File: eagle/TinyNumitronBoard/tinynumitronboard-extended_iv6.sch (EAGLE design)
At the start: 50 parts, among them IC1 74LS595D

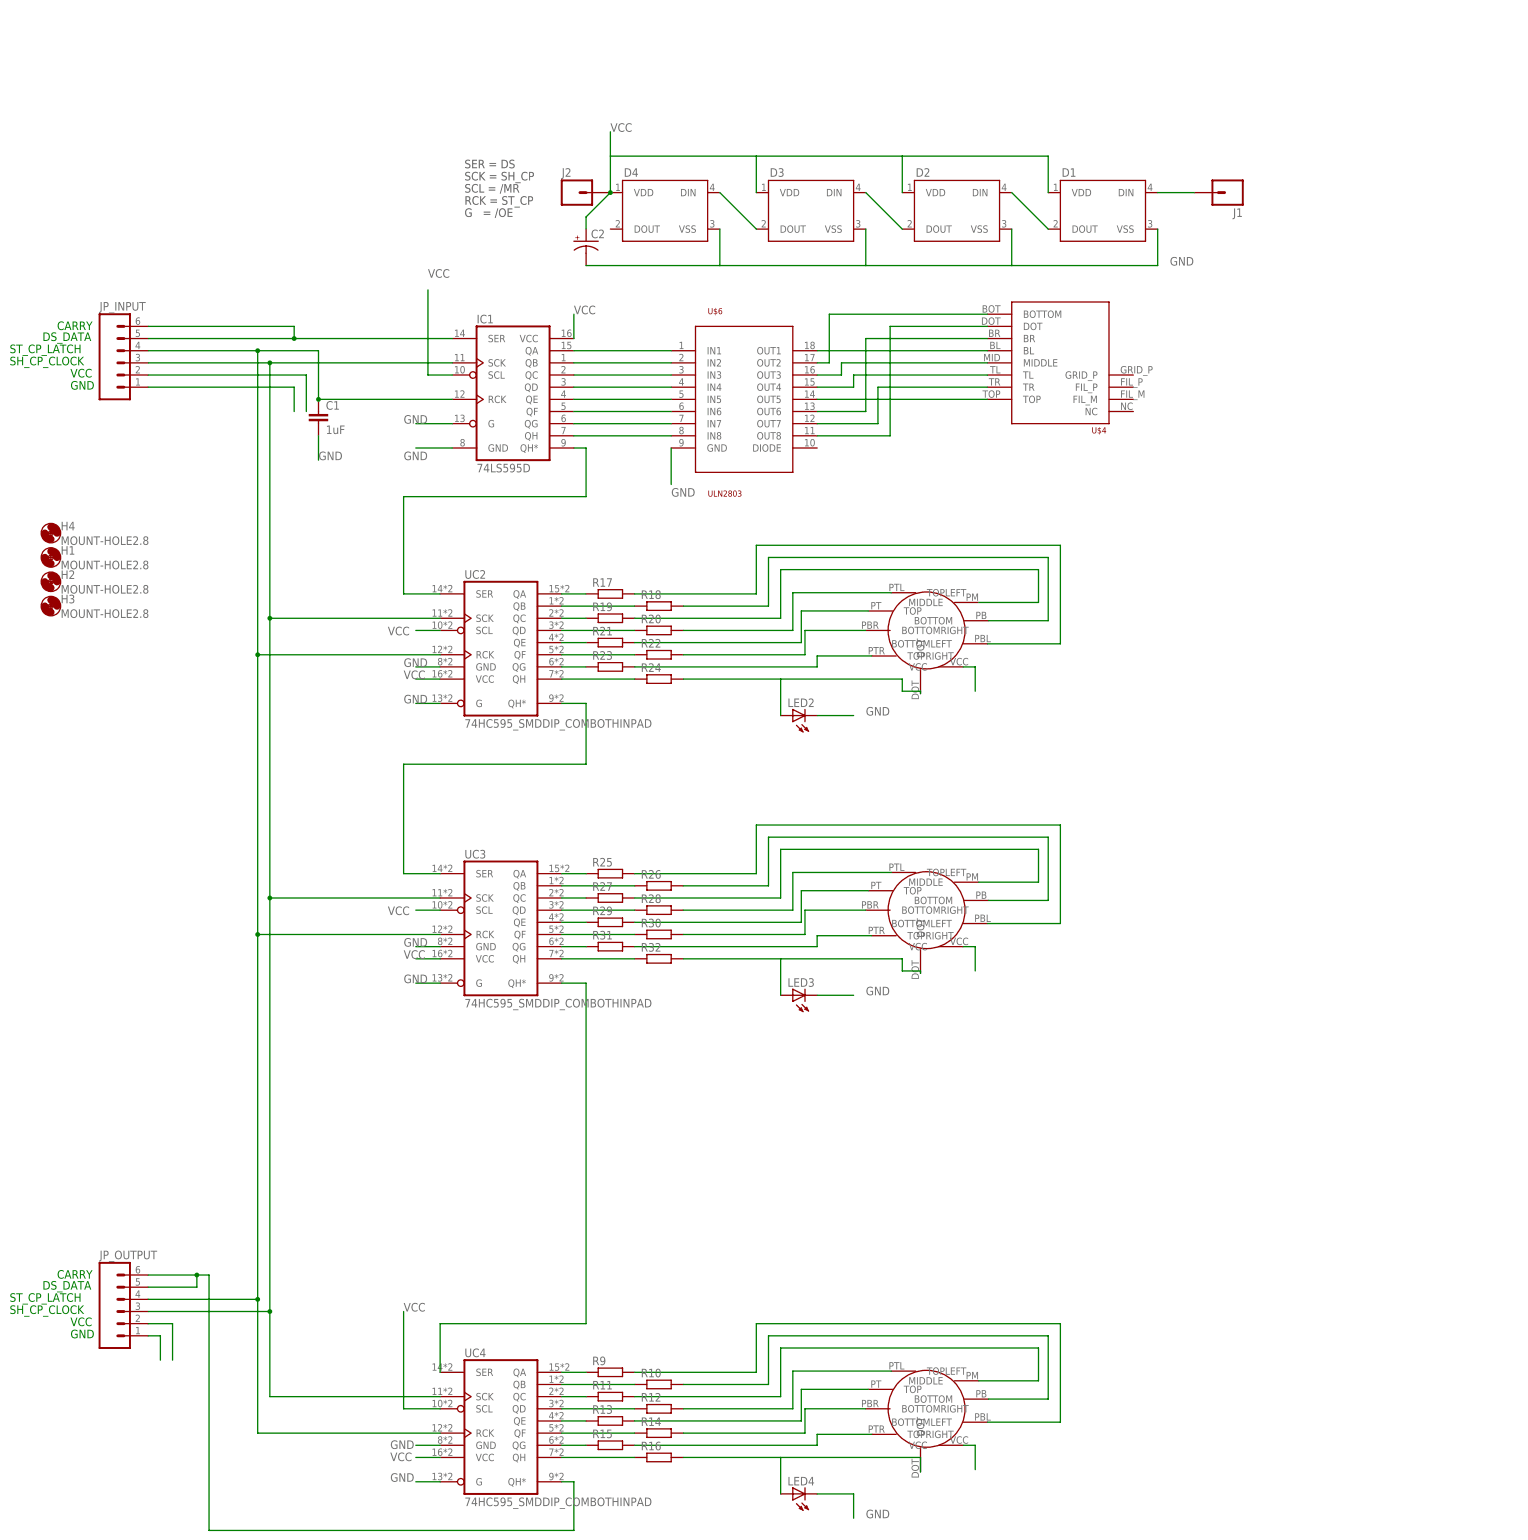
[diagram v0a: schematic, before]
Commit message: IV6 board dev continued.
Before taking some leap on placement. Schematics are ok minus final
review.
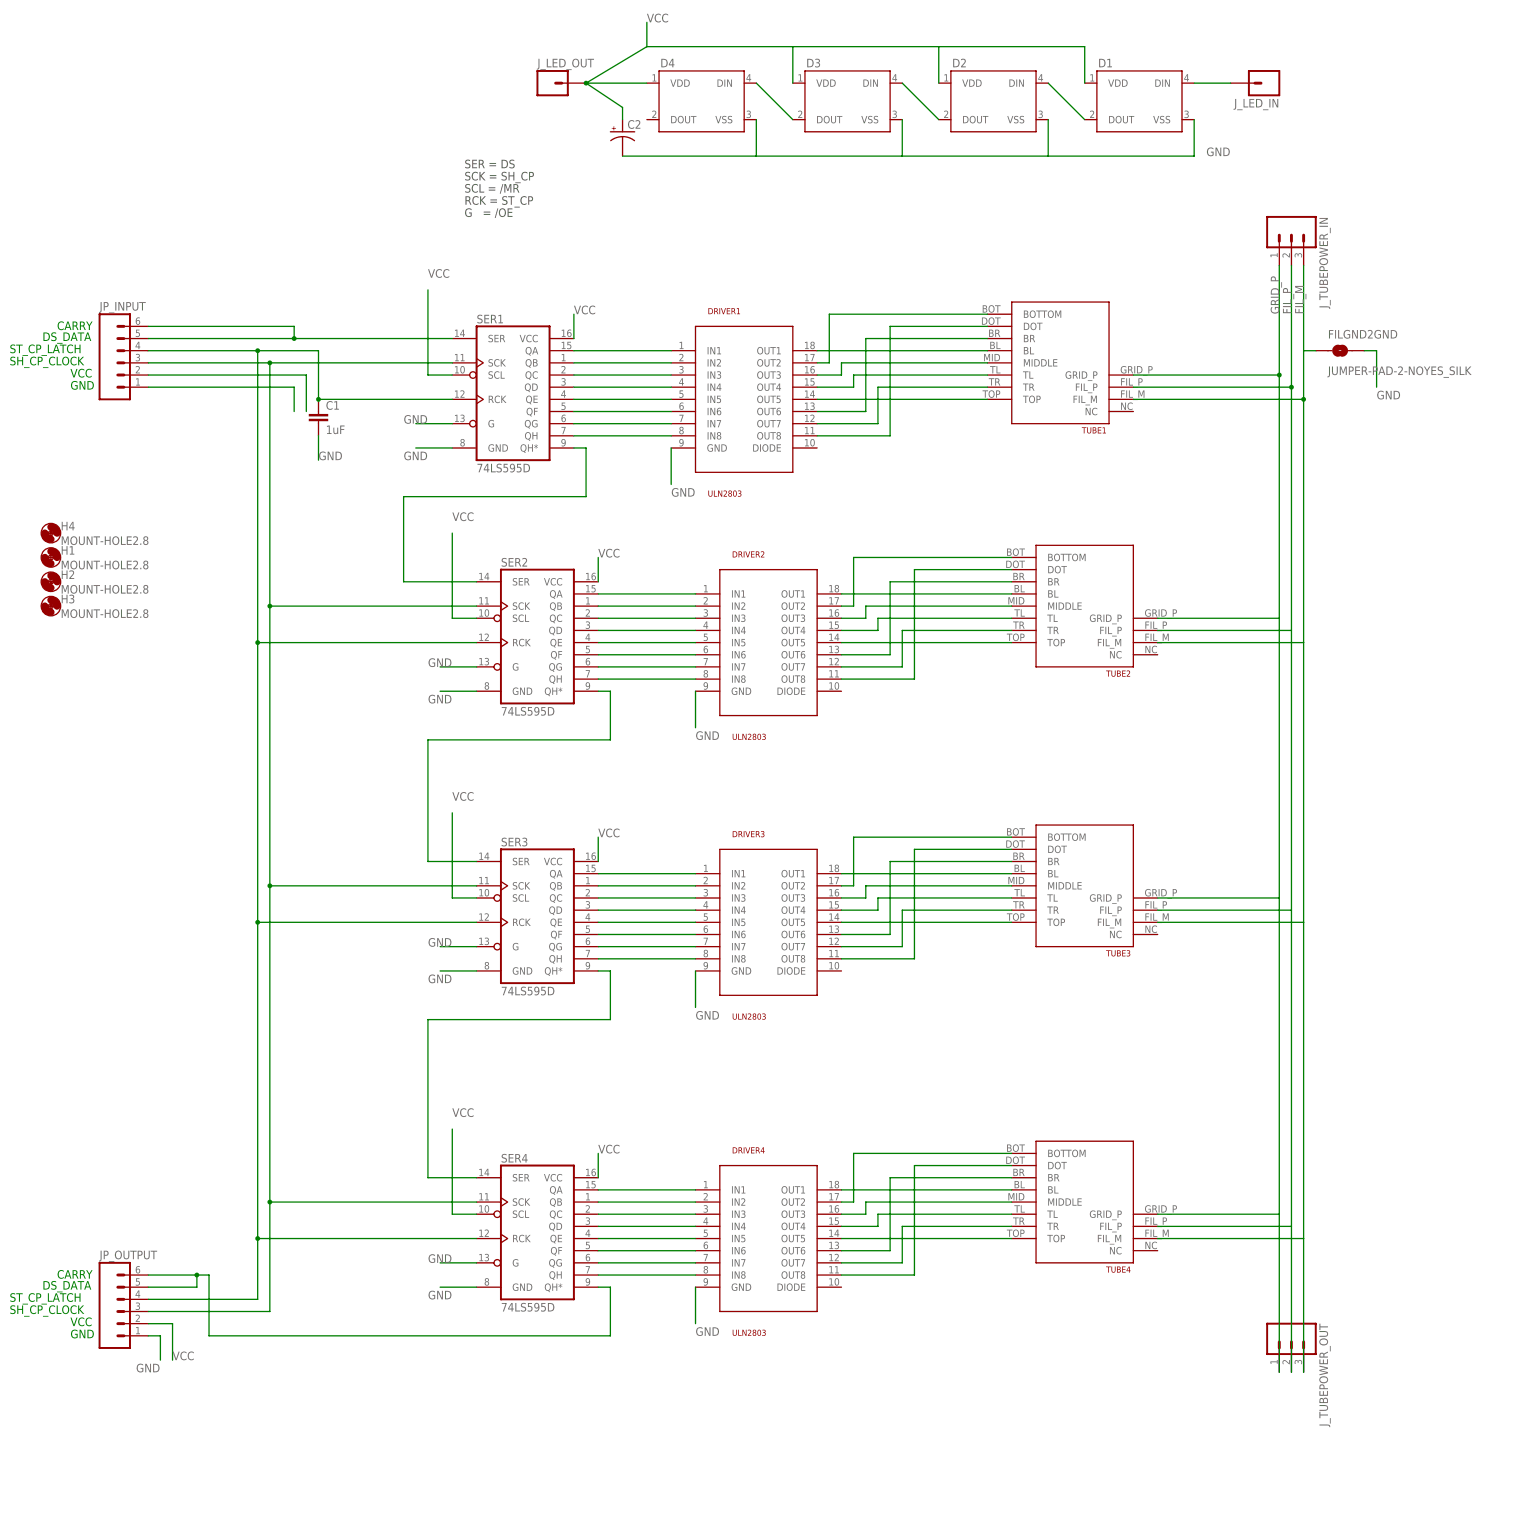
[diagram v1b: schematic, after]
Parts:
- removed J1, J2: (no value), SparkFun-Connectors:M01NOSILK-KIT
- removed LED2, LED3, LED4: (no value), led:LEDKA-3528ASYC
- removed R10, R11, R12, R13, R14, R15, R16, R17, R18, R19, R20, R21, R22, R23, R24, R25, R26, R27, R28, R29, R30, R31, R32, R9: (no value), resistor:R-EU_R1206
- removed U$2, U$5, U$7: IV16TINY_NUMITRON, kalshagar:IV16TINY_NUMITRON
- removed UC2, UC3, UC4: 74HC595_SMDDIP_COMBOTHINPAD, kalshagar:74HC595_SMDDIP_COMBOTHINPAD
- added DRIVER2, DRIVER3, DRIVER4: ULN2803, uln2803:ULN2803
- added FILGND2GND: JUMPER-PAD-2-NOYES_SILK, SparkFun-Passives:JUMPER-PAD-2-NOYES_SILK
- added J_LED_IN, J_LED_OUT: (no value), SparkFun-Connectors:M01NOSILK-KIT
- added J_TUBEPOWER_IN, J_TUBEPOWER_OUT: (no value), SparkFun-Connectors:M03LOCK
- added SER2, SER3, SER4: 74LS595D, SparkFun-DigitalIC:74LS595D
- added TUBE2, TUBE3, TUBE4: IV6_NUMITRONLARGE, kalshagar:IV6_NUMITRONLARGE
- C1: device resistor:C-EU050-024X044 -> resistor:C-EUC1206
- renumbered IC1 to SER1, U$4 to TUBE1, U$6 to DRIVER1
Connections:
- removed net N$20: R9.2, U$2.BOTTOMLEFT
- removed net N$22: JP_OUTPUT.5, JP_OUTPUT.6, UC4.QH*
- removed net N$75: R31.1, UC3.QG
- removed net N$76: R32.1, UC3.QH
- removed net N$77: LED3.A, R32.2, U$7.DOT
- removed net N$78: UC3.QH*, UC4.SER
- new net FIL_M: FILGND2GND.1, J_TUBEPOWER_IN.3, J_TUBEPOWER_OUT.3, TUBE1.FIL_M, TUBE2.FIL_M, TUBE3.FIL_M, TUBE4.FIL_M
- new net FIL_P: J_TUBEPOWER_IN.2, J_TUBEPOWER_OUT.2, TUBE1.FIL_P, TUBE2.FIL_P, TUBE3.FIL_P, TUBE4.FIL_P
- new net GRID_P: J_TUBEPOWER_IN.1, J_TUBEPOWER_OUT.1, TUBE1.GRID_P, TUBE2.GRID_P, TUBE3.GRID_P, TUBE4.GRID_P
- new net N$13: SER2.QH*, SER3.SER
- new net N$14: DRIVER2.OUT1, TUBE2.BL
- new net N$16: DRIVER2.OUT2, TUBE2.BOTTOM
- new net N$17: DRIVER2.OUT3, TUBE2.MIDDLE
- new net N$60: DRIVER3.OUT3, TUBE3.MIDDLE
- new net N$61: DRIVER3.OUT4, TUBE3.TL
- net GND: now also DRIVER2.GND, DRIVER3.GND, DRIVER4.GND, FILGND2GND.2, SER2.G, SER2.GND, SER3.G, SER3.GND, SER4.G, SER4.GND; no longer LED2.C, LED3.C, LED4.C, UC2.G, UC2.GND, UC3.G, UC3.GND, UC4.G, UC4.GND
- net N$12: now also J_LED_IN.1; no longer J1.1
- net N$21: now also JP_OUTPUT.5, JP_OUTPUT.6, SER4.QH*; no longer R10.2, U$2.BOTTOM
- net N$23: now also SER2.SER; no longer UC2.SER
- net N$24: now also DRIVER4.OUT1, TUBE4.BL; no longer R11.2, U$2.MIDDLE
- net N$25: now also DRIVER4.OUT2, TUBE4.BOTTOM; no longer R12.2, U$2.TOPLEFT
- net N$26: now also DRIVER4.OUT3, TUBE4.MIDDLE; no longer R13.2, U$2.TOP
- net N$27: now also DRIVER4.OUT4, TUBE4.TL; no longer R14.2, U$2.BOTTOMRIGHT
- net N$28: now also DRIVER4.OUT5, TUBE4.TOP; no longer R15.2, U$2.TOPRIGHT
- net N$29: now also DRIVER4.OUT6, TUBE4.BR; no longer R9.1, UC4.QA
- net N$30: now also DRIVER4.OUT7, TUBE4.TR; no longer R10.1, UC4.QB
- net N$31: now also DRIVER4.OUT8, TUBE4.DOT; no longer R11.1, UC4.QC
- net N$32: now also DRIVER4.IN1, SER4.QA; no longer R12.1, UC4.QD
- net N$33: now also DRIVER4.IN2, SER4.QB; no longer R13.1, UC4.QE
- net N$34: now also DRIVER4.IN3, SER4.QC; no longer R14.1, UC4.QF
- net N$35: now also DRIVER4.IN4, SER4.QD; no longer R15.1, UC4.QG
- net N$36: now also DRIVER4.IN5, SER4.QE; no longer R16.1, UC4.QH
- net N$37: now also DRIVER4.IN6, SER4.QF; no longer LED4.A, R16.2, U$2.DOT
- net N$39: now also DRIVER2.OUT4, TUBE2.TL; no longer R17.2, U$5.BOTTOMLEFT
- net N$40: now also DRIVER2.OUT5, TUBE2.TOP; no longer R18.2, U$5.BOTTOM
- net N$41: now also DRIVER2.OUT6, TUBE2.BR; no longer R19.2, U$5.MIDDLE
- net N$42: now also DRIVER2.OUT7, TUBE2.TR; no longer R20.2, U$5.TOPLEFT
- net N$43: now also DRIVER2.OUT8, TUBE2.DOT; no longer R21.2, U$5.TOP
- net N$44: now also DRIVER2.IN1, SER2.QA; no longer R22.2, U$5.BOTTOMRIGHT
- net N$45: now also DRIVER2.IN2, SER2.QB; no longer R23.2, U$5.TOPRIGHT
- net N$46: now also DRIVER2.IN3, SER2.QC; no longer R17.1, UC2.QA
- net N$47: now also DRIVER2.IN4, SER2.QD; no longer R18.1, UC2.QB
- net N$48: now also DRIVER2.IN5, SER2.QE; no longer R19.1, UC2.QC
- net N$49: now also DRIVER2.IN6, SER2.QF; no longer R20.1, UC2.QD
- net N$50: now also DRIVER2.IN7, SER2.QG; no longer R21.1, UC2.QE
- net N$51: now also DRIVER2.IN8, SER2.QH; no longer R22.1, UC2.QF
- net N$52: now also DRIVER4.IN7, SER4.QG; no longer R23.1, UC2.QG
- net N$53: now also SER3.QH*, SER4.SER; no longer R24.1, UC2.QH
- net N$54: now also DRIVER3.OUT1, TUBE3.BL; no longer LED2.A, R24.2, U$5.DOT
- net N$58: now also DRIVER3.OUT2, TUBE3.BOTTOM; no longer UC2.QH*, UC3.SER
- net N$62: now also DRIVER3.OUT5, TUBE3.TOP; no longer R25.2, U$7.BOTTOMLEFT
- net N$63: now also DRIVER3.OUT6, TUBE3.BR; no longer R26.2, U$7.BOTTOM
- net N$64: now also DRIVER3.OUT7, TUBE3.TR; no longer R27.2, U$7.MIDDLE
- net N$65: now also DRIVER3.OUT8, TUBE3.DOT; no longer R28.2, U$7.TOPLEFT
- net N$66: now also DRIVER3.IN1, SER3.QA; no longer R29.2, U$7.TOP
- net N$67: now also DRIVER3.IN2, SER3.QB; no longer R30.2, U$7.BOTTOMRIGHT
- net N$68: now also DRIVER3.IN3, SER3.QC; no longer R31.2, U$7.TOPRIGHT
- net N$69: now also DRIVER3.IN4, SER3.QD; no longer R25.1, UC3.QA
- net N$70: now also DRIVER3.IN5, SER3.QE; no longer R26.1, UC3.QB
- net N$71: now also DRIVER3.IN6, SER3.QF; no longer R27.1, UC3.QC
- net N$72: now also DRIVER3.IN7, SER3.QG; no longer R28.1, UC3.QD
- net N$73: now also DRIVER3.IN8, SER3.QH; no longer R29.1, UC3.QE
- net N$74: now also DRIVER4.IN8, SER4.QH; no longer R30.1, UC3.QF
- net RCK: now also SER2.RCK, SER3.RCK, SER4.RCK; no longer UC2.RCK, UC3.RCK, UC4.RCK
- net SCK: now also SER2.SCK, SER3.SCK, SER4.SCK; no longer UC2.SCK, UC3.SCK, UC4.SCK
- net VCC: now also J_LED_OUT.1, SER2.SCL, SER2.VCC, SER3.SCL, SER3.VCC, SER4.SCL, SER4.VCC; no longer J2.1, U$2.VCC, U$5.VCC, U$7.VCC, UC2.SCL, UC2.VCC, UC3.SCL, UC3.VCC, UC4.SCL, UC4.VCC
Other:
- moved on the sheet: C2, D1, D2, D3, D4
